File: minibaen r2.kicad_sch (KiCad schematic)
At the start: 121 parts, among them SW1 SW_Push, SW2 RotaryEncoder_Switch, U1 ATmega32U2-A, U2 PRTR5V0U2X, Y1 Crystal_GND24_Small

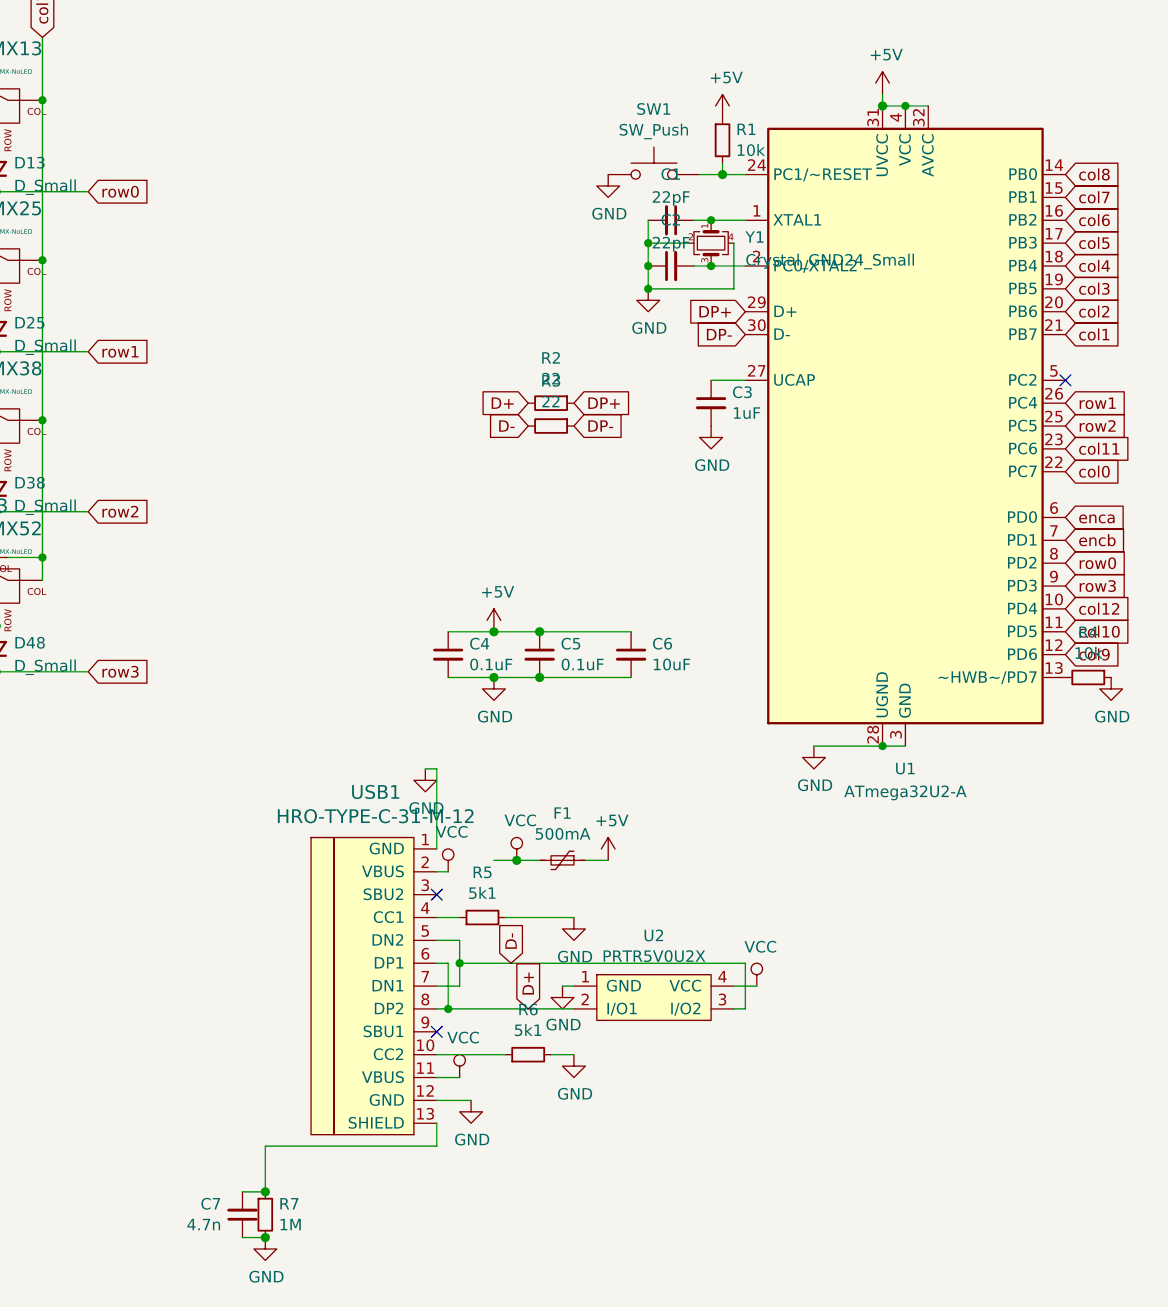
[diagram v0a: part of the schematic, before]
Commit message: add
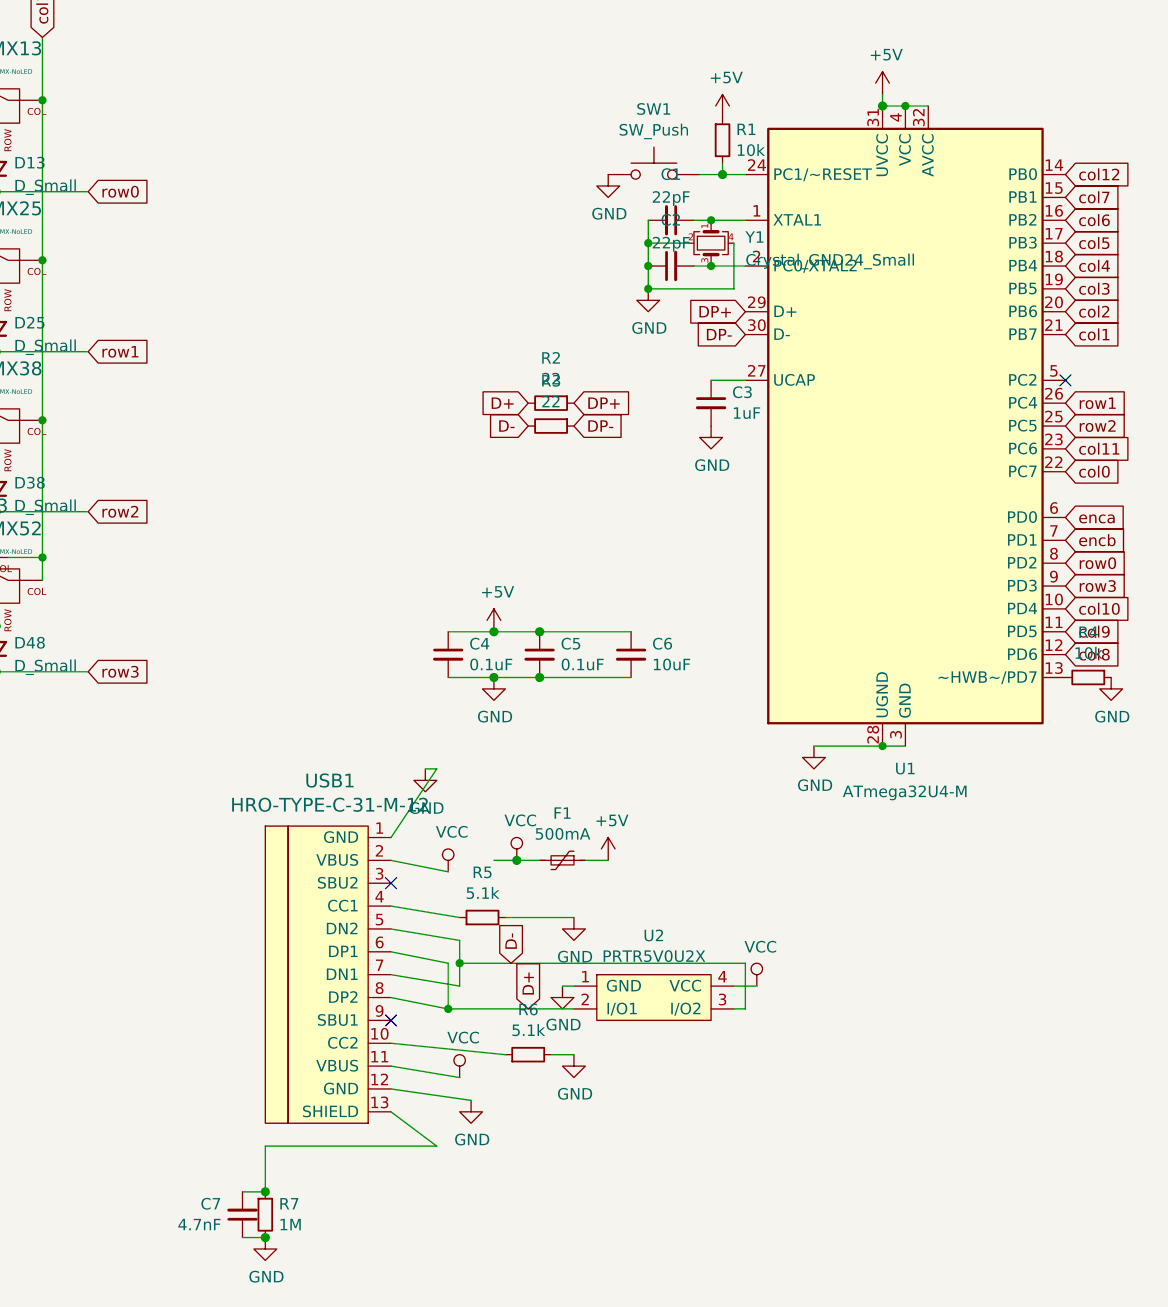
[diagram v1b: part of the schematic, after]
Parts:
- C7: value 4.7n -> 4.7nF
- R5, R6: value 5k1 -> 5.1k
- SW1: footprint Connector_PinHeader_2.54mm:PinHeader_1x02_P2.54mm_Vertical -> Button_Switch_SMD:SW_Push_SPST_NO_Alps_SKRK
- U1: value ATmega32U2-A -> ATmega32U4-M; footprint Package_QFP:TQFP-32_7x7mm_P0.8mm -> Package_DFN_QFN:QFN-44-1EP_7x7mm_P0.5mm_EP5.2x5.2mm
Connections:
- net col10: now also U1.10 (PD4); no longer U1.11 (PD5)
- net col12: now also U1.14 (PB0); no longer U1.10 (PD4)
- net col8: now also U1.12 (PD6); no longer U1.14 (PB0)
- net col9: now also U1.11 (PD5); no longer U1.12 (PD6)
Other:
- moved on the sheet: USB1
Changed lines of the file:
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@@
   (no_connect (at 127.635 55.88))
   (no_connect (at 280.67 64.77))
-  (no_connect (at 210.82 121.92))
-  (no_connect (at 210.82 137.16))
+  (no_connect (at 205.74 120.65))
+  (no_connect (at 205.74 135.89))
   (wire (pts (xy 227.33 118.11) (xy 229.87 118.11))
     (stroke (width 0) (type solid) (color 0 0 0 0))
@@
     (stroke (width 0) (type solid) (color 0 0 0 0))
   )
-  (wire (pts (xy 210.82 142.24) (xy 213.36 142.24))
+  (wire (pts (xy 205.74 140.97) (xy 213.36 142.24))
     (stroke (width 0) (type solid) (color 0 0 0 0))
   )
@@
     (stroke (width 0) (type solid) (color 0 0 0 0))
   )
-  (wire (pts (xy 210.82 107.95) (xy 210.82 116.84))
+  (wire (pts (xy 210.82 107.95) (xy 205.74 115.57))
     (stroke (width 0) (type solid) (color 0 0 0 0))
   )
@@
     (stroke (width 0) (type solid) (color 0 0 0 0))
   )
-  (wire (pts (xy 210.82 147.32) (xy 210.82 149.86))
+  (wire (pts (xy 205.74 146.05) (xy 210.82 149.86))
     (stroke (width 0) (type solid) (color 0 0 0 0))
   )
@@
     (stroke (width 0) (type solid) (color 0 0 0 0))
   )
-  (wire (pts (xy 210.82 119.38) (xy 212.09 119.38))
+  (wire (pts (xy 205.74 118.11) (xy 212.09 119.38))
     (stroke (width 0) (type solid) (color 0 0 0 0))
   )
@@
     (stroke (width 0) (type solid) (color 0 0 0 0))
   )
-  (wire (pts (xy 210.82 124.46) (xy 213.36 124.46))
+  (wire (pts (xy 205.74 123.19) (xy 213.36 124.46))
     (stroke (width 0) (type solid) (color 0 0 0 0))
   )
@@
     (stroke (width 0) (type solid) (color 0 0 0 0))
   )
-  (wire (pts (xy 210.82 144.78) (xy 214.63 144.78))
+  (wire (pts (xy 205.74 143.51) (xy 214.63 144.78))
     (stroke (width 0) (type solid) (color 0 0 0 0))
   )
@@
     (stroke (width 0) (type solid) (color 0 0 0 0))
   )
-  (wire (pts (xy 210.82 139.7) (xy 218.44 139.7))
+  (wire (pts (xy 205.74 138.43) (xy 218.44 139.7))
     (stroke (width 0) (type solid) (color 0 0 0 0))
   )
@@
     (stroke (width 0) (type solid) (color 0 0 0 0))
   )
-  (wire (pts (xy 210.82 127) (xy 213.36 127))
+  (wire (pts (xy 205.74 125.73) (xy 213.36 127))
     (stroke (width 0) (type solid) (color 0 0 0 0))
   )
-  (wire (pts (xy 212.09 134.62) (xy 210.82 134.62))
+  (wire (pts (xy 212.09 134.62) (xy 205.74 133.35))
     (stroke (width 0) (type solid) (color 0 0 0 0))
   )
@@
     (stroke (width 0) (type default) (color 0 0 0 0))
   )
-  (wire (pts (xy 213.36 132.08) (xy 210.82 132.08))
+  (wire (pts (xy 213.36 132.08) (xy 205.74 130.81))
     (stroke (width 0) (type solid) (color 0 0 0 0))
   )
@@
     (stroke (width 0) (type default) (color 0 0 0 0))
   )
-  (wire (pts (xy 210.82 129.54) (xy 212.09 129.54))
+  (wire (pts (xy 205.74 128.27) (xy 212.09 129.54))
     (stroke (width 0) (type solid) (color 0 0 0 0))
   )
@@
     )
   )
-  (global_label "col12" (shape input) (at 280.67 90.17 0) (fields_autoplaced)
+  (global_label "col12" (shape input) (at 280.67 41.91 0) (fields_autoplaced)
     (effects (font (size 1.27 1.27)) (justify left))
-    (property "Intersheet References" "${INTERSHEET_REFS}" (id 0) (at 288.405 90.0906 0)
+    (property "Intersheet References" "${INTERSHEET_REFS}" (id 0) (at 288.405 41.8306 0)
       (effects (font (size 1.27 1.27)) (justify left) hide)
     )
@@
     )
   )
-  (global_label "col9" (shape input) (at 280.67 95.25 0) (fields_autoplaced)
+  (global_label "col9" (shape input) (at 280.67 92.71 0) (fields_autoplaced)
     (effects (font (size 1.27 1.27)) (justify left))
-    (property "Intersheet References" "${INTERSHEET_REFS}" (id 0) (at 287.1955 95.1706 0)
+    (property "Intersheet References" "${INTERSHEET_REFS}" (id 0) (at 287.1955 92.6306 0)
       (effects (font (size 1.27 1.27)) (justify left) hide)
     )
@@
     )
   )
-  (global_label "col8" (shape input) (at 280.67 41.91 0) (fields_autoplaced)
+  (global_label "col8" (shape input) (at 280.67 95.25 0) (fields_autoplaced)
     (effects (font (size 1.27 1.27)) (justify left))
-    (property "Intersheet References" "${INTERSHEET_REFS}" (id 0) (at 287.1955 41.8306 0)
+    (property "Intersheet References" "${INTERSHEET_REFS}" (id 0) (at 287.1955 95.1706 0)
       (effects (font (size 1.27 1.27)) (justify left) hide)
     )
@@
     )
   )
-  (global_label "col10" (shape input) (at 280.67 92.71 0) (fields_autoplaced)
+  (global_label "col10" (shape input) (at 280.67 90.17 0) (fields_autoplaced)
     (effects (font (size 1.27 1.27)) (justify left))
-    (property "Intersheet References" "${INTERSHEET_REFS}" (id 0) (at 288.405 92.6306 0)
+    (property "Intersheet References" "${INTERSHEET_REFS}" (id 0) (at 288.405 90.0906 0)
       (effects (font (size 1.27 1.27)) (justify left) hide)
     )
@@
     (property "Reference" "SW1" (id 0) (at 234.95 34.671 0))
     (property "Value" "SW_Push" (id 1) (at 234.95 36.9824 0))
-    (property "Footprint" "Connector_PinHeader_2.54mm:PinHeader_1x02_P2.54mm_Vertical" (id 2) (at 234.95 36.83 0)
+    (property "Footprint" "Button_Switch_SMD:SW_Push_SPST_NO_Alps_SKRK" (id 2) (at 234.95 36.83 0)
       (effects (font (size 1.27 1.27)) hide)
     )
@@
     (pin "2")
   )
-  (symbol (lib_id "Type-C:HRO-TYPE-C-31-M-12") (at 208.28 130.81 0) (unit 1)
+  (symbol (lib_id "Type-C:HRO-TYPE-C-31-M-12") (at 203.2 129.54 0) (unit 1)
     (in_bom yes) (on_board yes)
-    (property "Reference" "USB1" (id 0) (at 204.0382 110.5662 0)
+    (property "Reference" "USB1" (id 0) (at 198.9582 109.2962 0)
       (effects (font (size 1.524 1.524)))
     )
-    (property "Value" "HRO-TYPE-C-31-M-12" (id 1) (at 204.0382 113.2586 0)
+    (property "Value" "HRO-TYPE-C-31-M-12" (id 1) (at 198.9582 111.9886 0)
       (effects (font (size 1.524 1.524)))
     )
-    (property "Footprint" "Type-C:HRO-TYPE-C-31-M-12" (id 2) (at 208.28 130.81 0)
+    (property "Footprint" "Type-C:HRO-TYPE-C-31-M-12" (id 2) (at 203.2 129.54 0)
       (effects (font (size 1.524 1.524)) hide)
     )
-    (property "Datasheet" "" (id 3) (at 208.28 130.81 0)
+    (property "Datasheet" "" (id 3) (at 203.2 129.54 0)
       (effects (font (size 1.524 1.524)) hide)
     )
@@
       (effects (font (size 1.27 1.27)) (justify right))
     )
-    (property "Value" "4.7n" (id 1) (at 186.8932 158.623 0)
+    (property "Value" "4.7nF" (id 1) (at 186.8932 158.623 0)
       (effects (font (size 1.27 1.27)) (justify right))
     )
@@
     (in_bom yes) (on_board yes)
     (property "Reference" "R5" (id 0) (at 215.9 119.4816 90))
-    (property "Value" "5k1" (id 1) (at 215.9 121.793 90))
+    (property "Value" "5.1k" (id 1) (at 215.9 121.793 90))
     (property "Footprint" "Resistor_SMD:R_0603_1608Metric" (id 2) (at 215.9 124.46 0)
       (effects (font (size 1.27 1.27)) hide)
@@
     (in_bom yes) (on_board yes)
     (property "Reference" "R6" (id 0) (at 220.98 134.7216 90))
-    (property "Value" "5k1" (id 1) (at 220.98 137.033 90))
+    (property "Value" "5.1k" (id 1) (at 220.98 137.033 90))
     (property "Footprint" "Resistor_SMD:R_0603_1608Metric" (id 2) (at 220.98 139.7 0)
       (effects (font (size 1.27 1.27)) hide)
@@
     (in_bom yes) (on_board yes) (fields_autoplaced)
     (property "Reference" "U1" (id 0) (at 262.89 107.95 0))
-    (property "Value" "ATmega32U2-A" (id 1) (at 262.89 110.49 0))
-    (property "Footprint" "Package_QFP:TQFP-32_7x7mm_P0.8mm" (id 2) (at 262.89 69.85 0)
+    (property "Value" "ATmega32U4-M" (id 1) (at 262.89 110.49 0))
+    (property "Footprint" "Package_DFN_QFN:QFN-44-1EP_7x7mm_P0.5mm_EP5.2x5.2mm" (id 2) (at 262.89 69.85 0)
       (effects (font (size 1.27 1.27) italic) hide)
     )
-    (property "Datasheet" "http://ww1.microchip.com/downloads/en/DeviceDoc/doc7799.pdf" (id 3) (at 262.89 69.85 0)
+    (property "Datasheet" "" (id 3) (at 262.89 69.85 0)
       (effects (font (size 1.27 1.27)) hide)
     )
@@
     )
     (path "/00000000-0000-0000-0000-00005fb89313"
-      (reference "C7") (unit 1) (value "4.7n") (footprint "Capacitor_SMD:C_0603_1608Metric")
+      (reference "C7") (unit 1) (value "4.7nF") (footprint "Capacitor_SMD:C_0603_1608Metric")
     )
     (path "/4096bf41-3908-453c-b16b-52b72a81b7a4"
@@
     )
     (path "/00000000-0000-0000-0000-00005fc48136"
-      (reference "R5") (unit 1) (value "5k1") (footprint "Resistor_SMD:R_0603_1608Metric")
+      (reference "R5") (unit 1) (value "5.1k") (footprint "Resistor_SMD:R_0603_1608Metric")
     )
     (path "/00000000-0000-0000-0000-00005fc49d19"
-      (reference "R6") (unit 1) (value "5k1") (footprint "Resistor_SMD:R_0603_1608Metric")
+      (reference "R6") (unit 1) (value "5.1k") (footprint "Resistor_SMD:R_0603_1608Metric")
     )
     (path "/00000000-0000-0000-0000-00005fb8883d"
@@
     )
     (path "/00000000-0000-0000-0000-00005faca656"
-      (reference "SW1") (unit 1) (value "SW_Push") (footprint "Connector_PinHeader_2.54mm:PinHeader_1x02_P2.54mm_Vertical")
+      (reference "SW1") (unit 1) (value "SW_Push") (footprint "Button_Switch_SMD:SW_Push_SPST_NO_Alps_SKRK")
     )
     (path "/29392f04-ea5c-48c3-8fe0-a41e8589c2b7"
@@
     )
     (path "/8541e986-2b2b-4942-8c66-0b6939dd52db"
-      (reference "U1") (unit 1) (value "ATmega32U2-A") (footprint "Package_QFP:TQFP-32_7x7mm_P0.8mm")
+      (reference "U1") (unit 1) (value "ATmega32U4-M") (footprint "Package_DFN_QFN:QFN-44-1EP_7x7mm_P0.5mm_EP5.2x5.2mm")
     )
     (path "/a143f620-ffcd-428f-be64-b671165c8969"
